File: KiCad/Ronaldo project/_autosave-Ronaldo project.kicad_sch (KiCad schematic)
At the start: 24 parts, among them J1 Power, J2 Program, M1 Motor_DC, SW1 Switch, SW2 Reset, SW3 SW_Push, SW4 SW_Push, SW5 SW_Push, U1 ATmega328P-P, U2 AMS1117-5.0, U3 L293D, Y1 16MHz

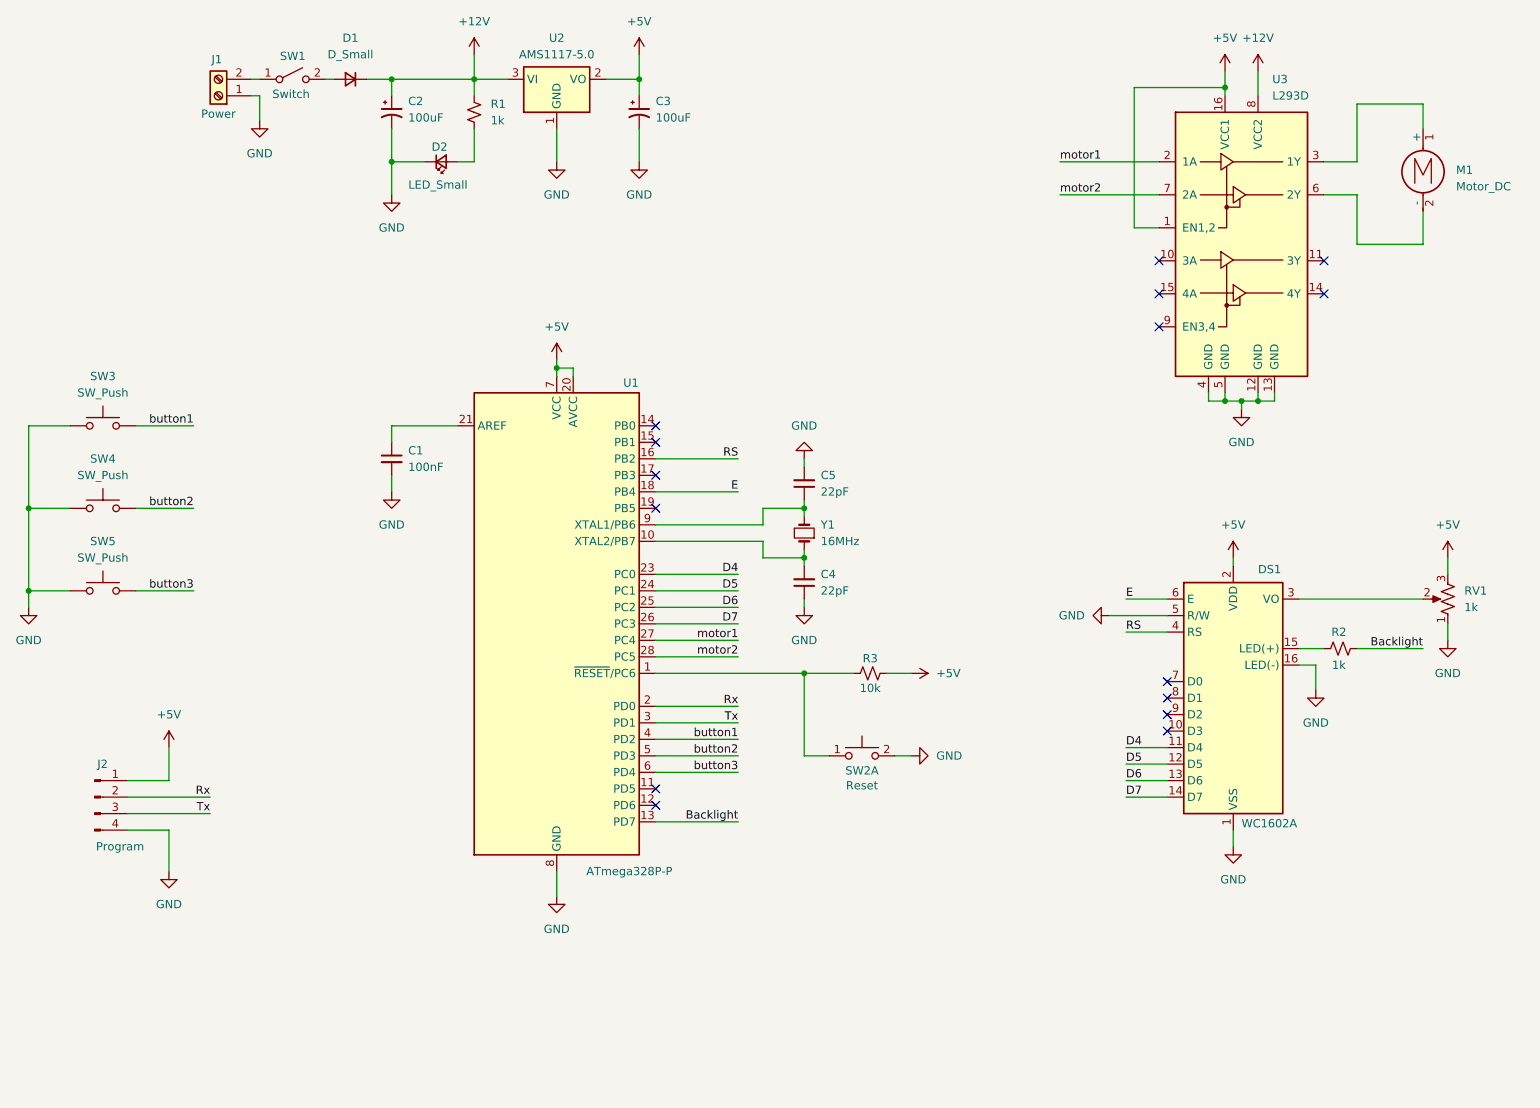
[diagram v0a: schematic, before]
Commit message: Changes
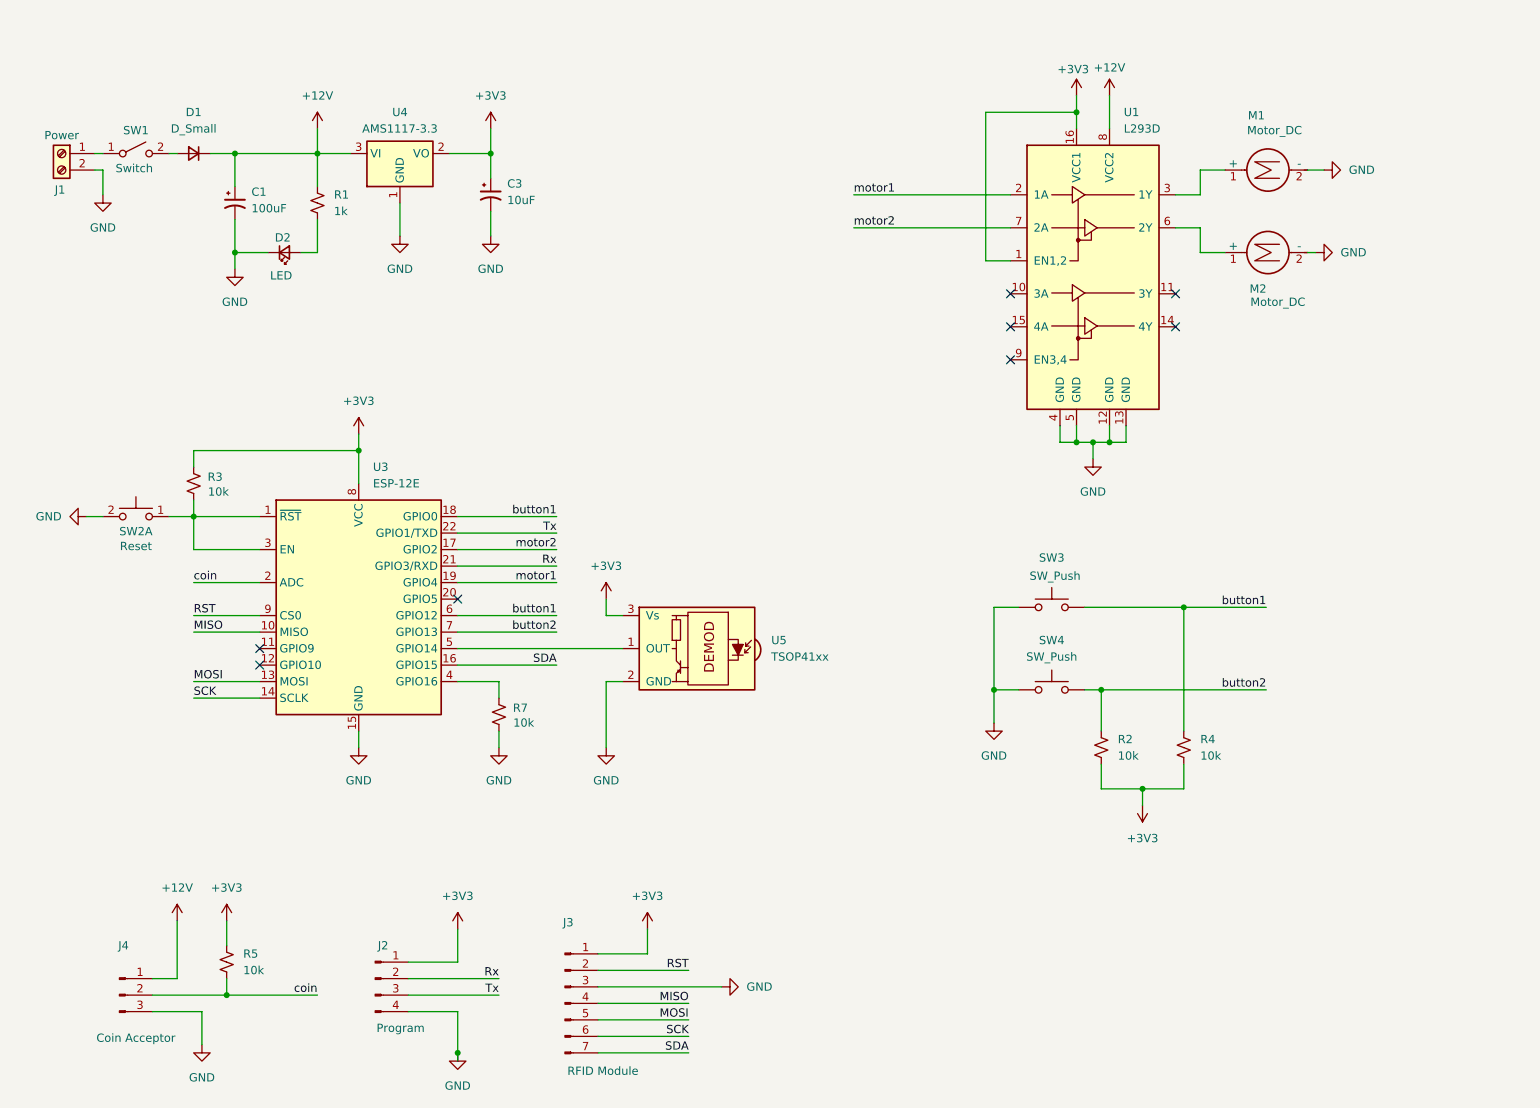
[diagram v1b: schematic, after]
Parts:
- removed C1: 100nF, Capacitor_THT:C_Disc_D3.0mm_W1.6mm_P2.50mm, symbol Device:C_Small
- removed C2: 100uF, Capacitor_THT:CP_Radial_D5.0mm_P2.50mm, symbol Device:C_Polarized_Small_US
- removed C4, C5: 22pF, Capacitor_THT:C_Disc_D3.0mm_W1.6mm_P2.50mm, symbol Device:C_Small
- removed DS1: WC1602A, Display:WC1602A, symbol Display_Character:WC1602A
- removed RV1: 1k, Potentiometer_THT:Potentiometer_Runtron_RM-065_Vertical, symbol Device:R_Potentiometer_US
- removed SW5: SW_Push, TestPoint:TestPoint_2Pads_Pitch2.54mm_Drill0.8mm, symbol Switch:SW_Push
- removed U1: ATmega328P-P, Package_DIP:DIP-28_W7.62mm_Socket_LongPads, symbol MCU_Microchip_ATmega:ATmega328P-P
- removed U2: AMS1117-5.0, Package_TO_SOT_SMD:SOT-223-3_TabPin2, symbol Regulator_Linear:AMS1117-5.0
- removed U3: L293D, Package_DIP:DIP-16_W7.62mm_Socket_LongPads, symbol Driver_Motor:L293D
- removed Y1: 16MHz, Crystal:Crystal_HC50_Vertical, symbol Device:Crystal_Small
- added C1: 100uF, Capacitor_THT:CP_Radial_D5.0mm_P2.50mm, symbol Device:C_Polarized_Small_US
- added J3: RFID Module, Connector_PinHeader_2.54mm:PinHeader_1x07_P2.54mm_Vertical, symbol Connector:Conn_01x07_Pin
- added J4: Coin Acceptor, Connector_PinHeader_2.54mm:PinHeader_1x03_P2.54mm_Vertical, symbol Connector:Conn_01x03_Pin
- added M2: Motor_DC, TerminalBlock:TerminalBlock_bornier-2_P5.08mm, symbol Motor:Motor_DC
- added R4, R5, R7: 10k, Resistor_THT:R_Axial_DIN0207_L6.3mm_D2.5mm_P10.16mm_Horizontal, symbol Device:R_Small_US
- added U1: L293D, Package_DIP:DIP-16_W7.62mm, symbol Driver_Motor:L293D
- added U3: ESP-12E, RF_Module:ESP-12E, symbol RF_Module:ESP-12E
- added U4: AMS1117-3.3, Package_TO_SOT_SMD:SOT-223-3_TabPin2, symbol Regulator_Linear:AMS1117-3.3
- added U5: TSOP41xx, OptoDevice:Vishay_MOLD-3Pin, symbol Interface_Optical:TSOP41xx
- C3: value 100uF -> 10uF
- D2: value LED_Small -> LED
- R2: value 1k -> 10k
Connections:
- net +5V is gone; now on net +3V3: C3.1, J2.1 (Pin_1), R3.2
- net Backlight is gone; now on net button2: R2.2
- net +12V: now also C1.1, J4.1 (Pin_1), U1.8 (VCC2), U4.3 (VI)
- net GND: now also J1.2 (Pin_2), M1.2 (-), C1.2, J3.3 (Pin_3), J4.3 (Pin_3), M2.2 (-), R7.1, U1.12 (GND), U1.13 (GND), U1.4 (GND), U1.5 (GND), U3.15 (GND), U4.1 (GND), U5.2 (GND); no longer J1.1 (Pin_1)
- net Rx: now also U3.21 (GPIO3/RXD)
- net Tx: now also U3.22 (GPIO1/TXD)
- net button1: now also R4.2, U3.18 (GPIO0), U3.6 (GPIO12)
- net button2: now also U3.7 (GPIO13)
- net motor1: now also U1.2 (1A), U3.19 (GPIO4)
- net motor2: now also U1.7 (2A), U3.17 (GPIO2)
- net at R3.1, SW2.1 (C): now also U3.1 (~{RST}), U3.3 (EN)
- net at M1.1 (+): now also U1.3 (1Y)
- net +3V3: now reaches R2.1
- net +3V3: now also J3.1 (Pin_1), R4.1, R5.2, U1.1 (EN1,2), U1.16 (VCC1), U3.8 (VCC), U4.2 (VO), U5.3 (Vs)
- net at SW1.1 (A): now also J1.1 (Pin_1); no longer J1.2 (Pin_2)
- new net: M2.1 (+), U1.6 (2Y)
- new net: U3.5 (GPIO14), U5.1 (OUT)
- new net: R7.2, U3.4 (GPIO16)
- new net MISO: J3.4 (Pin_4), U3.10 (MISO)
- new net MOSI: J3.5 (Pin_5), U3.13 (MOSI)
- new net RST: J3.2 (Pin_2), U3.9 (CS0)
- new net SCK: J3.6 (Pin_6), U3.14 (SCLK)
- new net SDA: J3.7 (Pin_7), U3.16 (GPIO15)
- new net coin: J4.2 (Pin_2), R5.1, U3.2 (ADC)
- no-connect marks 15 -> 8
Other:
- company: (none) -> University of Dar es salaam (UDSM)
- title: (none) -> SMART PAYMENT SYSTEM INTERGRATED WITH AN AUTOMATIC TEA/COFFEE MAKING MACHINE
